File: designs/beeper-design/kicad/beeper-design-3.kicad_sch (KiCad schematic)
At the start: 37 parts, among them J1 TC2030-IDC-NL, J6 10103594-0001LF, U1 DA14705-00000HZ2, U2 AT25FF321A-UUN-T, U7 TPD4S012DRYR

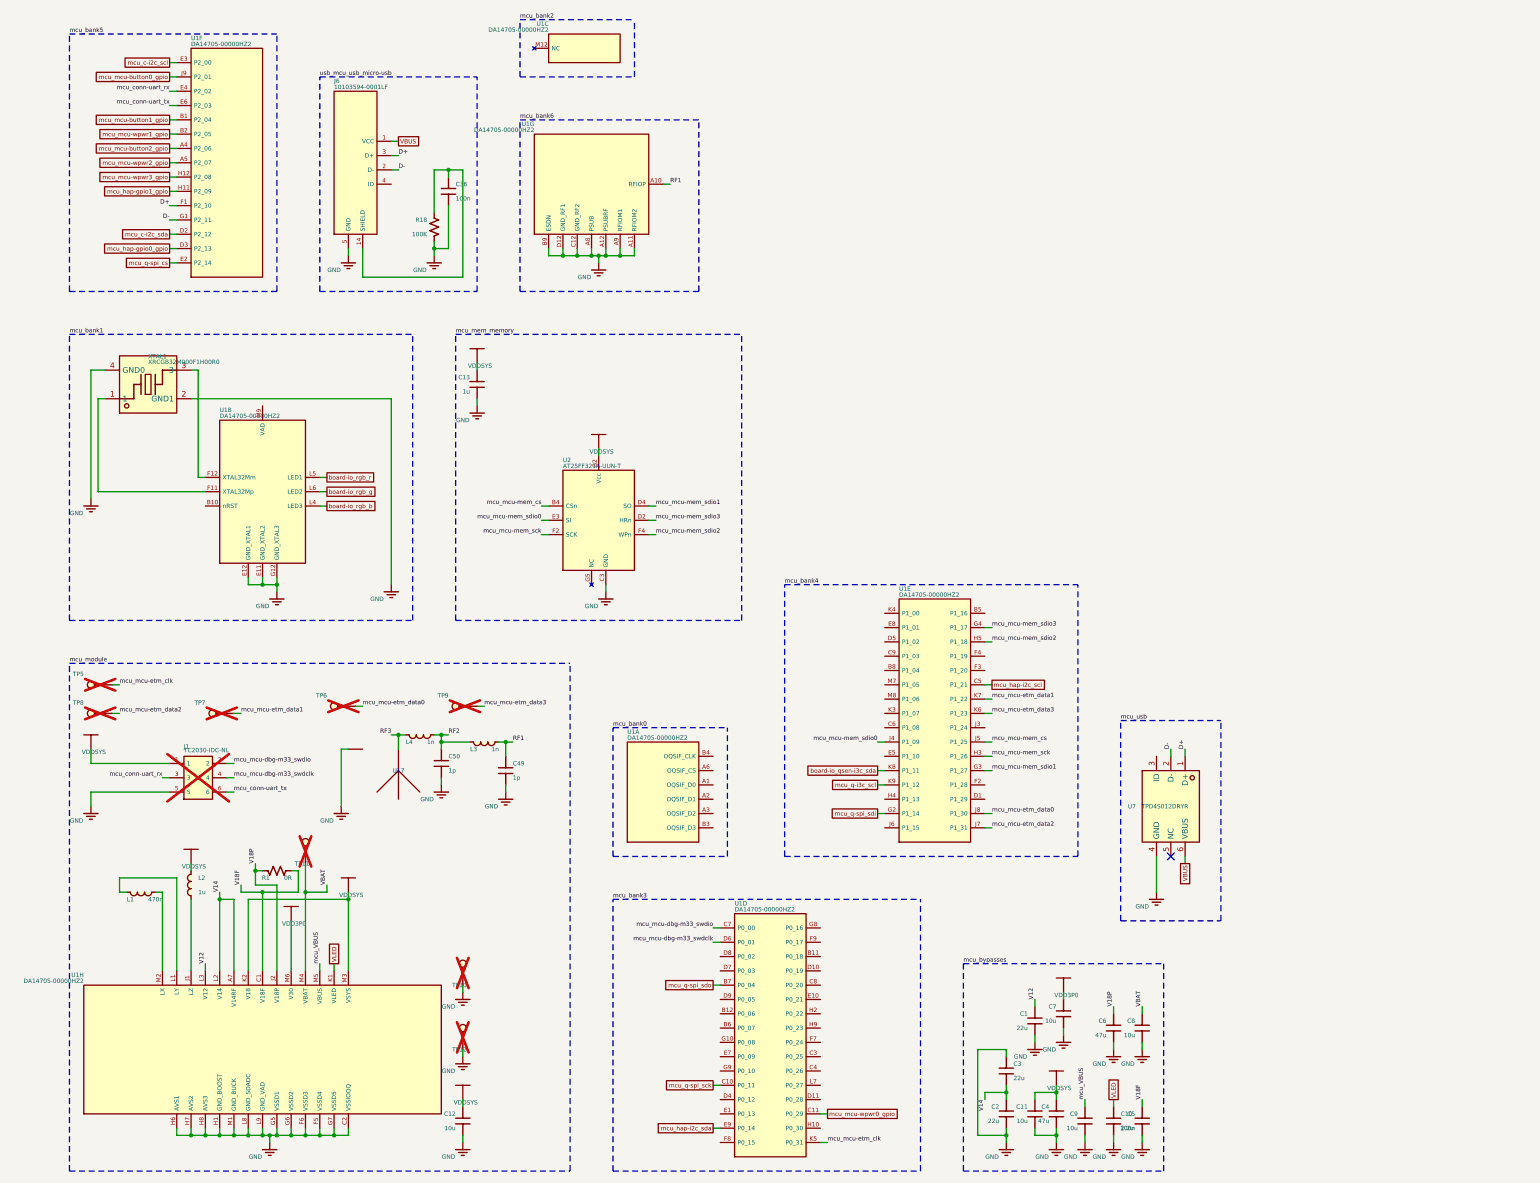
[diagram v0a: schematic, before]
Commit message: post export, had to munge sch
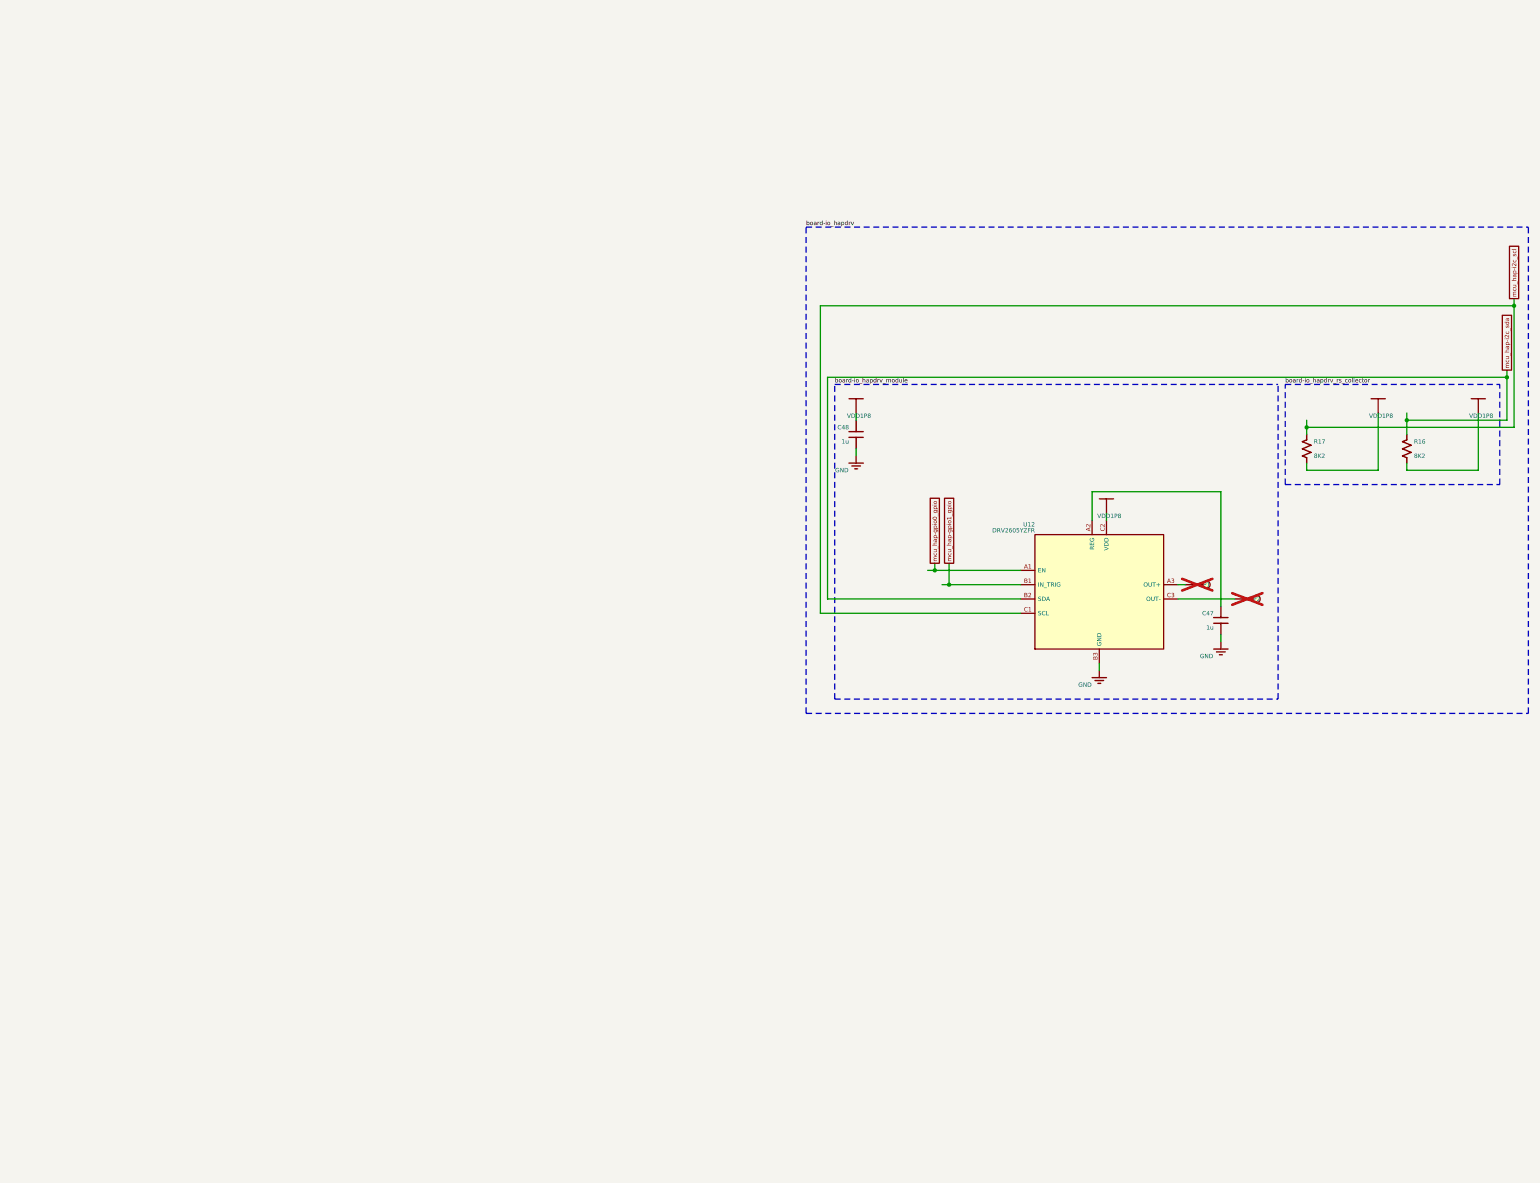
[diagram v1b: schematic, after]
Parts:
- removed C1: 22u, beeper-design:Pkg0603, symbol C86295_2
- removed C10: 2.2u, beeper-design:Pkg0201_11, symbol C318539
- removed C11: 10u, beeper-design:Pkg0402_1, symbol C962143_1
- removed C12: 10u, beeper-design:Pkg0402, symbol C962143
- removed C13: 1u, beeper-design:Pkg0201_27, symbol C76935_7
- removed C2: 22u, beeper-design:Pkg0603_1, symbol C86295
- removed C3: 22u, beeper-design:Pkg0603_2, symbol C86295_1
- removed C36: 100n, beeper-design:Pkg0201_24, symbol my_capacitor_3
- removed C4: 47u, beeper-design:Pkg0805_1, symbol my_capacitor_5
- removed C49: 1p, beeper-design:Pkg0201_32, symbol C277491
- removed C5: 100n, beeper-design:Pkg0201, symbol my_capacitor_8
- removed C50: 1p, beeper-design:Pkg0201_2, symbol C277491_1
- removed C6: 47u, beeper-design:Pkg0805, symbol my_capacitor_1
- removed C7: 10u, beeper-design:Pkg0402_2, symbol C962143_2
- removed C8: 10u, beeper-design:Pkg0402_4, symbol C962143_4
- removed C9: 10u, beeper-design:Pkg0402_9, symbol C962143_5
- removed J1: TC2030-IDC-NL, beeper-design:TC2030_IDC_NL_FOOTPRINT, symbol component
- removed J6: 10103594-0001LF, beeper-design:AMPHENOL_10103594_0001LF, symbol AMPHENOL_10103594_0001LF
- removed L1: 470n, beeper-design:Pkg0603_3, symbol C275359
- removed L2: 1u, beeper-design:Pkg0402_7, symbol C516791
- removed L3: 1n, beeper-design:Pkg0201_40, symbol C2041448_1
- removed L4: 1n, beeper-design:Pkg0201_9, symbol C2041448
- removed R1: 0R, beeper-design:Pkg0201_18, symbol C106228
- removed R18: 100K, beeper-design:Pkg0201_13, symbol C106230
- removed TP10, TP11, TP12, TP5, TP6, TP7, TP8, TP9: (no value), beeper-design:SMD_TESTPT, symbol smd_testpoint_cmp
- removed U1: DA14705-00000HZ2, beeper-design:LP, symbol DA14705
- removed U17: (no value), beeper-design:Pkg_2450AT18D0100_STD_R_1, symbol Sym2450AT18D0100
- removed U2: AT25FF321A-UUN-T, beeper-design:WLCSP_12, symbol AT25FF321A_UUN_T
- removed U7: TPD4S012DRYR, beeper-design:SON_6_L1_5_W1_0_P0_50_BL, symbol C96506
- removed XTAL1: XRCGB32M000F1H00R0, beeper-design:CRYSTAL_SMD_4P_L2_0_W1_6_BL_1, symbol C880116
- added C47: 1u, beeper-design:Pkg0201_40, symbol C76935_11
- added C48: 1u, beeper-design:Pkg0201_6, symbol C76935_2
- added R16, R17: 8K2, beeper-design:Pkg0201_20, symbol my_resistor_6
- added TP1, TP2: (no value), beeper-design:SMD_TESTPT, symbol smd_testpoint_cmp
- added U12: DRV2605YZFR, beeper-design:LP_8, symbol DRV2605YZFR
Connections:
- net GND: now also C47.1, C48.1, U12.B3 (GND)
- net mcu_hap-gpio0_gpio: now also U12.A1 (EN)
- net mcu_hap-gpio1_gpio: now also U12.B1 (IN_TRIG)
- net mcu_hap-i2c_scl: now also R17.1, U12.C1 (SCL)
- net mcu_hap-i2c_sda: now also R16.1, U12.B2 (SDA)
- new net: TP1.p, U12.A3 (OUT+)
- new net: C47.2, U12.A2 (REG)
- new net: TP2.p, U12.C3 (OUT-)
- new net VDD1P8: C48.2, R16.2, R17.2, U12.C2 (VDD)
- no-connect marks 1 -> 0
